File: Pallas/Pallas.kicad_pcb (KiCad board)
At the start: 2 copper layers, 467.5 x 140 mm, 263 parts, among them J1 OLED, J2 RGB_LED, Q1 IRLML6344TRPbF, SW00 SW_PUSH, SW01 SW_PUSH, SW010 SW_PUSH, SW011 SW_PUSH, SW012 SW_PUSH, SW013 SW_PUSH, SW014 SW_PUSH, SW02 SW_PUSH, SW03 SW_PUSH, SW04 SW_PUSH, SW05 SW_PUSH, SW06 SW_PUSH, SW07 SW_PUSH, SW08 SW_PUSH, SW09 SW_PUSH, SW10 SW_PUSH, SW11 SW_PUSH, SW110 SW_PUSH, SW111 SW_PUSH, SW112 SW_PUSH, SW113 SW_PUSH, SW114 SW_PUSH, SW12 SW_PUSH, SW13 SW_PUSH, SW14 SW_PUSH, SW15 SW_PUSH, SW16 SW_PUSH, SW17 SW_PUSH, SW18 SW_PUSH, SW19 SW_PUSH, SW20 SW_PUSH, SW21 SW_PUSH, SW210 SW_PUSH, SW211 SW_PUSH, SW212 SW_PUSH, SW213 SW_PUSH, SW214 SW_PUSH, SW22 SW_PUSH, SW23 SW_PUSH, SW24 SW_PUSH, SW25 SW_PUSH, SW26 SW_PUSH, SW27 SW_PUSH, SW28 SW_PUSH, SW29 SW_PUSH, SW30 SW_PUSH, SW31 SW_PUSH, SW310 SW_PUSH, SW311 SW_PUSH, SW312 SW_PUSH, SW313 SW_PUSH, SW314 SW_PUSH, SW32 SW_PUSH, SW33 SW_PUSH, SW34 SW_PUSH, SW35 SW_PUSH, SW36 SW_PUSH, SW37 SW_PUSH, SW38 SW_PUSH, SW39 SW_PUSH, SW40 SW_PUSH, SW41 SW_PUSH, SW410 SW_PUSH, SW411 SW_PUSH, SW412 SW_PUSH, SW413 SW_PUSH, SW414 SW_PUSH, SW42 SW_PUSH, SW43 SW_PUSH, SW44 SW_PUSH, SW45 SW_PUSH, SW46 SW_PUSH, SW47 SW_PUSH, SW48 SW_PUSH, SW49 SW_PUSH, U1 Elite-C

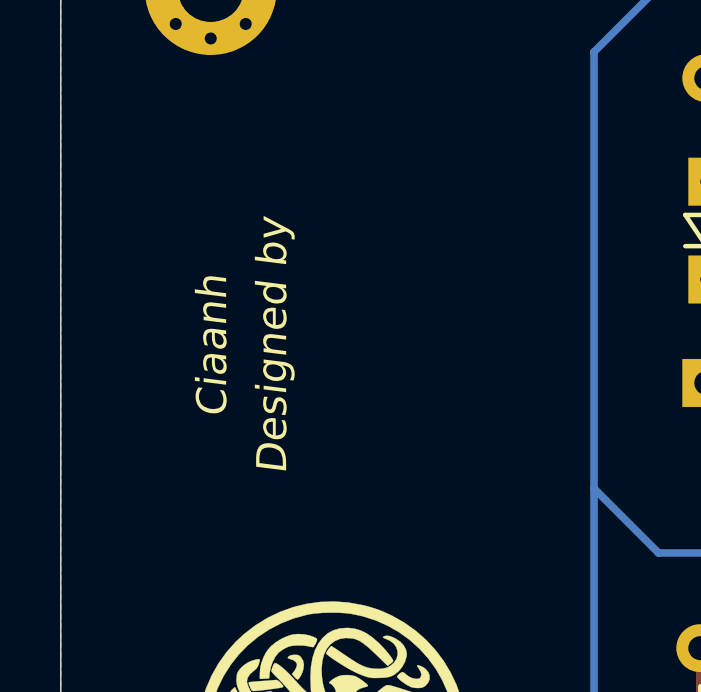
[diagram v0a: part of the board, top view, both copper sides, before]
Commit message: Fix issue with label design by
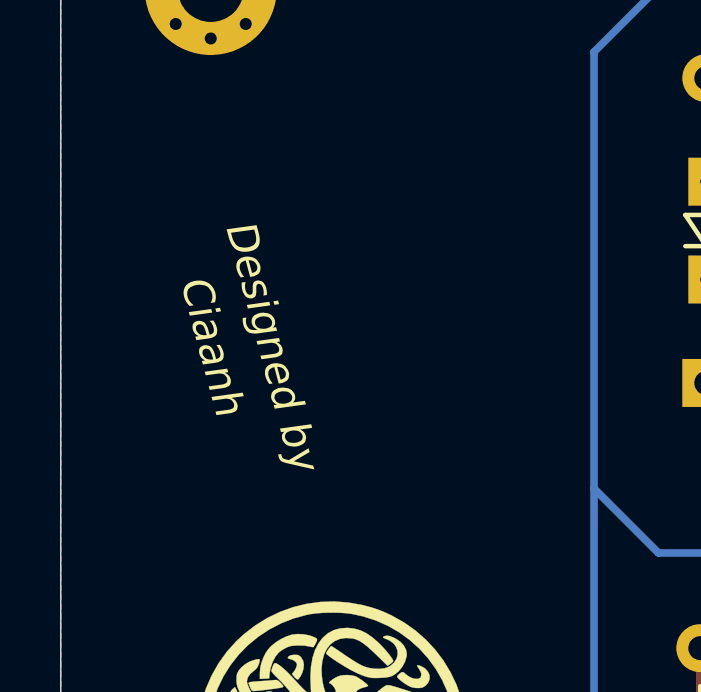
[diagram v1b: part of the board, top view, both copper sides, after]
